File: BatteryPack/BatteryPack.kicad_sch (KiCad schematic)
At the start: 31 parts, among them Q1 IRFR220NTRPBF, Q2 BC817-40, U2 ETA3000S2G, U3 ETA3000S2G, U4 ETA3000S2G

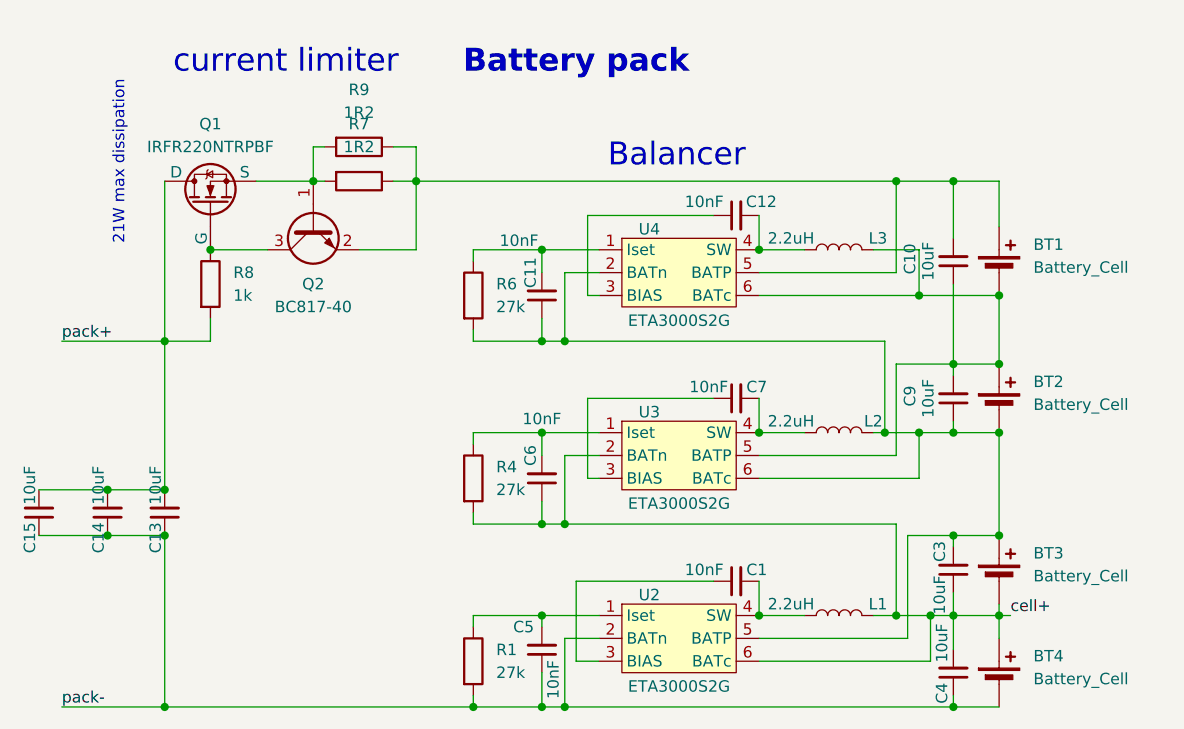
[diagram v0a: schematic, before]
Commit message: Add files via upload
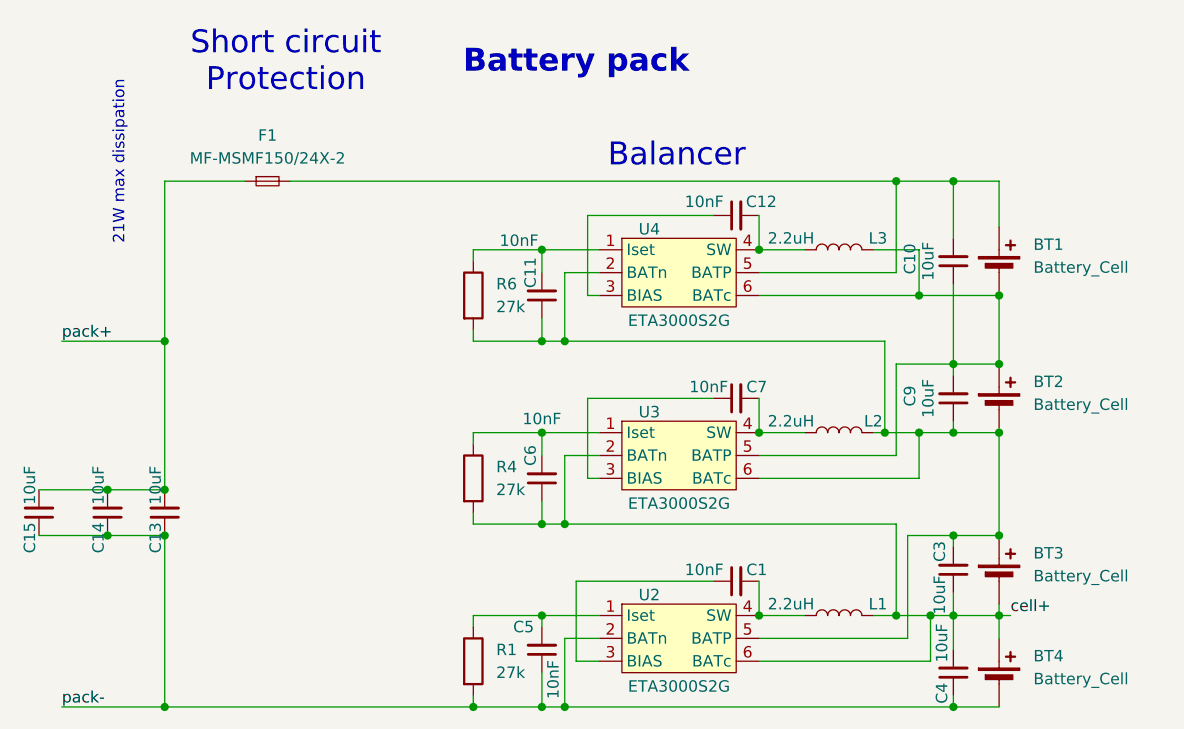
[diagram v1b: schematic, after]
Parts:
- removed Q1: IRFR220NTRPBF, Package_TO_SOT_SMD:TO-252-2, symbol Simulation_SPICE:NMOS
- removed Q2: BC817-40, Package_TO_SOT_SMD:SOT-23, symbol Transistor_BJT:Q_NPN_BEC
- removed R7, R9: 1R2, Resistor_SMD:R_1206_3216Metric_Pad1.30x1.75mm_HandSolder, symbol Device:R
- removed R8: 1k, Resistor_SMD:R_0603_1608Metric_Pad0.98x0.95mm_HandSolder, symbol Device:R
- added F1: MF-MSMF150/24X-2, Fuse:Fuse_1812_4532Metric_Pad1.30x3.40mm_HandSolder, symbol Device:Fuse_Small
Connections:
- net pack+: now also F1.1
- net at BT1.1 (+), C10.2, U4.5 (BATP): now also F1.2
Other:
- note added: "Short circuit Protection"
- note removed: "current limiter"
